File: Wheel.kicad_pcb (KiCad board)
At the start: 2 copper layers, 70.1 x 38.9 mm, 52 parts, among them J1 USB_C_Receptacle_USB2.0_16P, J2 Conn_01x06, J3 Conn_01x06, J4 Conn_01x06, J5 Conn_01x06, J6 Conn_01x03, J7 Conn_01x05, SW1 SW_Push, SW2 SW_Push, U1 STM32F407VGTx, U2 AMS1117-3.3, U3 MT6835

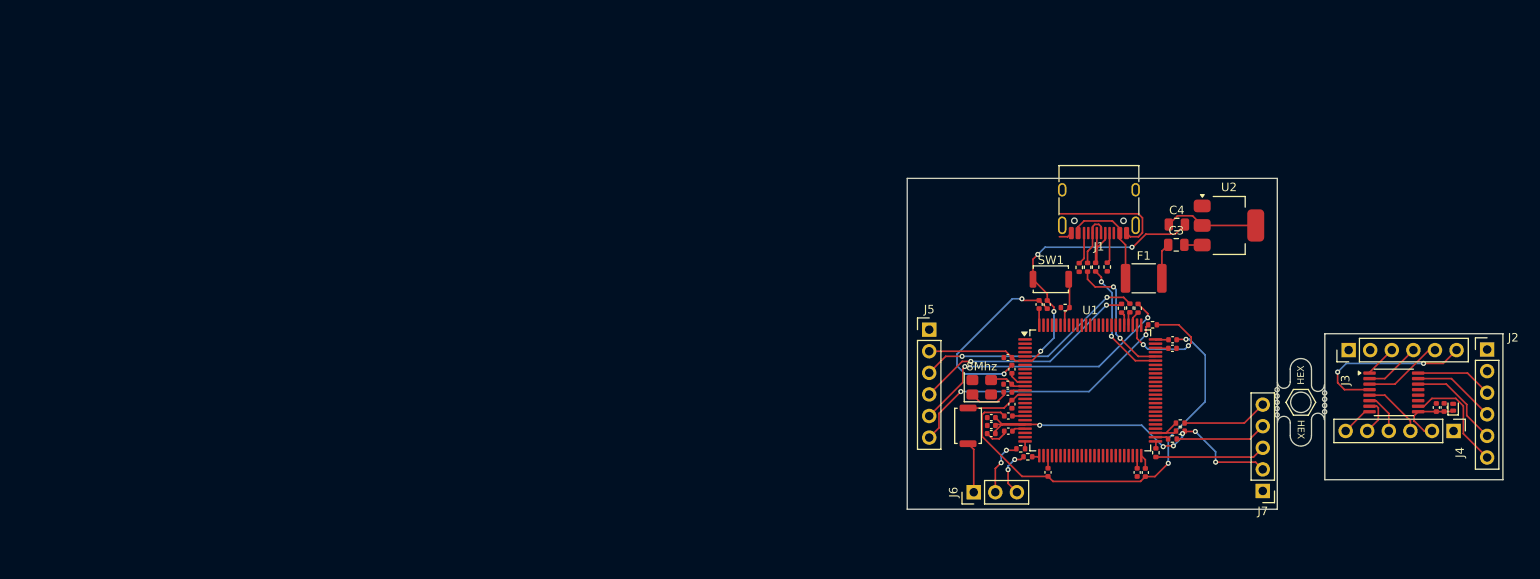
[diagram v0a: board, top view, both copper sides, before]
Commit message: Update
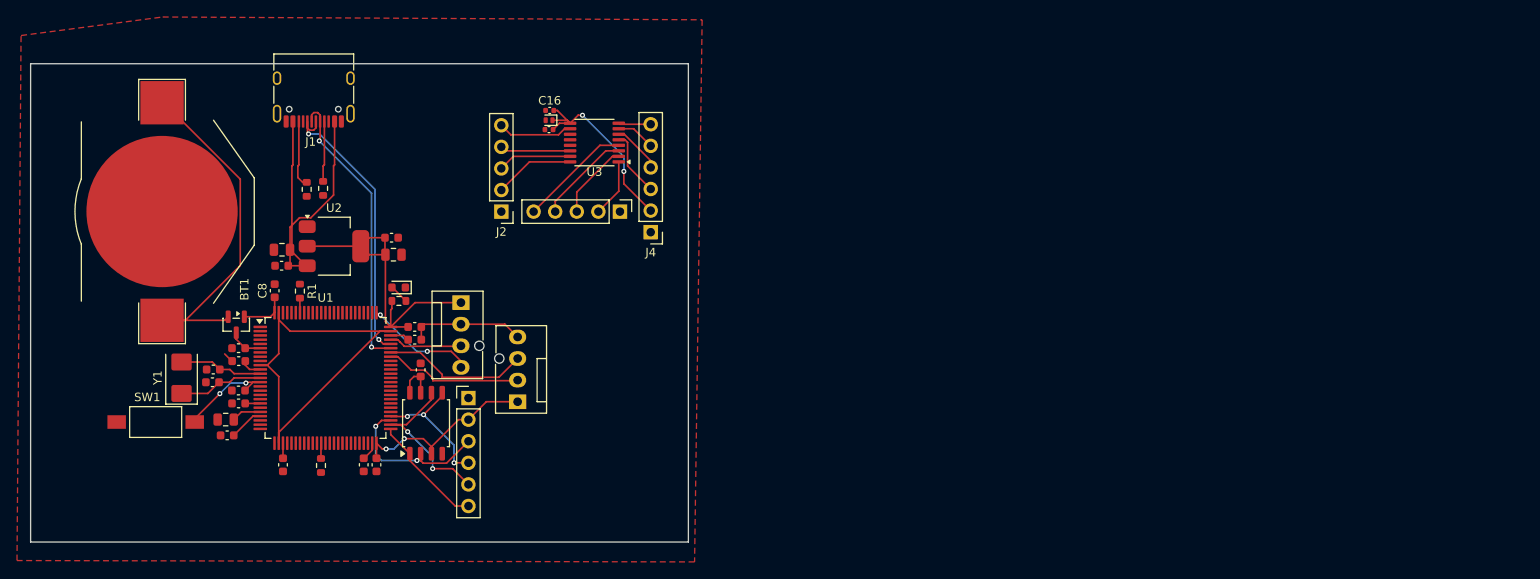
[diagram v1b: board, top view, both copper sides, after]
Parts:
- removed 8Mhz: Crystal_GND24, Crystal:Crystal_SMD_3225-4Pin_3.2x2.5mm
- removed F1: Polyfuse, Fuse:Fuse_1812_4532Metric
- removed MB5: 5.5mm, PCM_marbastlib-various:mousebites_5p5mm_easysnap
- removed R10, R11, R12, R13, R14: 100Ω, Resistor_SMD:R_0402_1005Metric
- removed R15: 10k, Resistor_SMD:R_0402_1005Metric
- removed R6, R7, R8, R9: 22Ω, Resistor_SMD:R_0402_1005Metric
- removed SW2: SW_Push, Button_Switch_SMD:SW_Push_SPST_NO_Alps_SKRK
- added BT1: Battery, Battery:BatteryHolder_Keystone_3002_1x2032, F.Cu at (77.3, 42.9)
- added D2: LED, LED_SMD:LED_0603_1608Metric, F.Cu at (105.1, 51.9)
- added D3: BAT54C, Package_TO_SOT_SMD:SOT-23, F.Cu at (86.0, 56.2)
- added U4: W25Q16JVSS, Package_SO:SOIC-8_5.3x5.3mm_P1.27mm, F.Cu at (108.3, 67.8)
- added Y1: 8MHz, Crystal:Crystal_SMD_5032-2Pin_5.0x3.2mm, F.Cu at (79.6, 62.5)
- C1, C2: value 2.2µF -> 104; footprint Capacitor_SMD:C_0402_1005Metric -> Capacitor_SMD:C_0603_1608Metric
- C10: value 100nF -> 2.2uF; footprint Capacitor_SMD:C_0402_1005Metric -> Capacitor_SMD:C_0603_1608Metric
- C11: value 4.7µF -> 2.2uF; footprint Capacitor_SMD:C_0402_1005Metric -> Capacitor_SMD:C_0603_1608Metric
- C12: value 0.1µF -> 106; footprint Capacitor_SMD:C_0402_1005Metric -> Capacitor_SMD:C_0805_2012Metric
- C13: value 27pf -> 104; footprint Capacitor_SMD:C_0402_1005Metric -> Capacitor_SMD:C_0603_1608Metric
- C14: value 27pf -> 106; footprint Capacitor_SMD:C_0402_1005Metric -> Capacitor_SMD:C_0805_2012Metric
- C17, C19: value 1µF -> 104; footprint Capacitor_SMD:C_0402_1005Metric -> Capacitor_SMD:C_0603_1608Metric
- C18: value 10nF -> 104; footprint Capacitor_SMD:C_0402_1005Metric -> Capacitor_SMD:C_0603_1608Metric
- C20: value 10nF -> 20P; footprint Capacitor_SMD:C_0402_1005Metric -> Capacitor_SMD:C_0603_1608Metric
- C21: value 100nF -> 20P; footprint Capacitor_SMD:C_0402_1005Metric -> Capacitor_SMD:C_0603_1608Metric
- C3: value 22µF -> 104; footprint Capacitor_SMD:C_0805_2012Metric -> Capacitor_SMD:C_0603_1608Metric
- C4: value 10µF -> 104; footprint Capacitor_SMD:C_0805_2012Metric -> Capacitor_SMD:C_0603_1608Metric
- C5, C6, C7, C8: value 100nF -> 104; footprint Capacitor_SMD:C_0402_1005Metric -> Capacitor_SMD:C_0603_1608Metric
- C9: value 100nF -> 106; footprint Capacitor_SMD:C_0402_1005Metric -> Capacitor_SMD:C_0805_2012Metric
- J1: value USB_C_Receptacle_USB2.0_16P -> USB_C_Receptacle_USB2.0_14P
- J2: value Conn_01x06 -> GND-A-B-Z-PWM; footprint Connector_PinHeader_2.54mm:PinHeader_1x06_P2.54mm_Vertical -> Connector_PinHeader_2.54mm:PinHeader_1x05_P2.54mm_Vertical
- J3: value Conn_01x06 -> CAL-W-V-U-GND; footprint Connector_PinHeader_2.54mm:PinHeader_1x06_P2.54mm_Vertical -> Connector_PinHeader_2.54mm:PinHeader_1x05_P2.54mm_Vertical
- J4: value Conn_01x06 -> J4(Pins 6-3)-VDDA(1)/3V3-GND
- J6: value Conn_01x03 -> Conn_01x04; footprint Connector_PinHeader_2.54mm:PinHeader_1x03_P2.54mm_Vertical -> Connector:FanPinHeader_1x04_P2.54mm_Vertical
- J7: value Conn_01x05 -> UART; footprint Connector_PinHeader_2.54mm:PinHeader_1x05_P2.54mm_Vertical -> Connector:FanPinHeader_1x04_P2.54mm_Vertical
- R1: value 5.1k -> 10k; footprint Resistor_SMD:R_0402_1005Metric -> Resistor_SMD:R_0603_1608Metric
- R2: footprint Resistor_SMD:R_0402_1005Metric -> Resistor_SMD:R_0603_1608Metric
- R3: value 20Ω -> 5.1k; footprint Resistor_SMD:R_0402_1005Metric -> Resistor_SMD:R_0603_1608Metric
- R4: value 20Ω -> 10K; footprint Resistor_SMD:R_0402_1005Metric -> Resistor_SMD:R_0603_1608Metric
- R5: value 10KΩ -> 510R; footprint Resistor_SMD:R_0402_1005Metric -> Resistor_SMD:R_0603_1608Metric
- SW1: footprint Button_Switch_SMD:SW_Push_SPST_NO_Alps_SKRK -> Button_Switch_SMD:SW_SPST_FSMSM
- moved J2 117.1 mm to (117.2, 42.9), turned to 180 degrees
- moved C4 112.4 mm to (86.3, 65.5), turned to 180 degrees
- moved C9 111.8 mm to (84.8, 67.4)
- moved D1 111.6 mm to (122.8, 32.2), turned to 180 degrees
- moved C3 111.2 mm to (86.3, 60.5), turned to 180 degrees
- moved C15 110.3 mm to (122.8, 33.3), turned to 0 degrees
- moved C16 110.0 mm to (122.9, 31.0), turned to 0 degrees
- moved SW1 106.7 mm to (76.5, 67.7)
- moved C1 106.2 mm to (86.3, 64.0), turned to 0 degrees
- moved U2 105.3 mm to (97.5, 47.0)
- moved C8 104.7 mm to (90.5, 52.2)
- moved U3 98.6 mm to (128.1, 34.8), turned to 180 degrees
- moved J4 97.3 mm to (134.8, 45.4), turned to 180 degrees
- moved C7 96.7 mm to (84.9, 69.3), turned to 180 degrees
- moved R1 95.0 mm to (93.5, 52.3)
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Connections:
- C1 pad 2: Net-(U1-VCAP_1) -> Net-(U1-NRST)
- C10 pad 1: Net-(C10-Pad1) -> GND
- C10 pad 2: Net-(C10-Pad2) -> Net-(U1-VCAP_1)
- C11 pad 1: +3V3 -> GND
- C11 pad 2: Net-(C10-Pad1) -> Net-(U1-VCAP_2)
- C12 pad 1: GND -> +5V
- C12 pad 2: Net-(U1-NRST) -> GND
- C13 pad 1: GND -> +5V
- C13 pad 2: Net-(U1-PH0) -> GND
- C14 pad 1: Net-(U1-PH1) -> VDDA(1)
- C14 pad 2: Net-(8Mhz1-Pad1) -> GND
- C15 pad 2: VCC -> VDDA(1)
- C16 pad 2: VCC -> VDDA(1)
- C17 pad 1: +3V3 -> VDDA(1)
- C18 pad 1: GND -> VBAT
- C18 pad 2: +3V3 -> GND
- C19 pad 1: Net-(C19-Pad1) -> GND
- C19 pad 2: Net-(U1-VDDA) -> Net-(U4-VCC)
- C2 pad 2: Net-(U1-VCAP_2) -> VDDA(1)
- C20 pad 1: +3V3 -> GND
- C20 pad 2: Net-(C19-Pad1) -> OSC_IN
- C21 pad 2: +3V3 -> OSC_OUT
- C3 pad 1: Net-(C3-Pad1) -> VDDA(1)
- C3 pad 2: Net-(U2-VI) -> GND
- C4 pad 1: Net-(U2-VO) -> VDDA(1)
- C4 pad 2: +3V3 -> GND
- C5 pad 1: Net-(C10-Pad1) -> VDDA(1)
- C5 pad 2: Net-(C5-Pad2) -> GND
- C6 pad 1: Net-(C10-Pad1) -> VDDA(1)
- C6 pad 2: Net-(C6-Pad2) -> GND
- C7 pad 1: Net-(C10-Pad1) -> VDDA(1)
- C7 pad 2: Net-(C7-Pad2) -> GND
- C8 pad 1: Net-(C10-Pad1) -> VDDA(1)
- C8 pad 2: Net-(C8-Pad2) -> GND
- C9 pad 1: Net-(C10-Pad1) -> VDDA(1)
- C9 pad 2: Net-(C9-Pad2) -> GND
- D1 pad 1: VCC -> VDDA(1)
- J1 pad A1: Net-(J1-GND-PadA1) -> GND
- J1 pad A12: Net-(J1-GND-PadA1) -> GND
- J1 pad A4: Net-(F1-Pad1) -> +5V
- J1 pad A6: D+ -> USB_DP
- J1 pad A7: D- -> USB_DM
- J1 pad A8: unconnected-(J1-SBU1-PadA8) -> (no net)
- J1 pad A9: Net-(F1-Pad1) -> +5V
- J1 pad B1: Net-(J1-GND-PadA1) -> GND
- J1 pad B12: Net-(J1-GND-PadA1) -> GND
- J1 pad B4: Net-(F1-Pad1) -> +5V
- J1 pad B6: D+ -> USB_DP
- J1 pad B7: D- -> USB_DM
- J1 pad B8: unconnected-(J1-SBU2-PadB8) -> (no net)
- J1 pad B9: Net-(F1-Pad1) -> +5V
- J1 pad SH: unconnected-(J1-SHIELD-PadSH) -> GND
- J2 pad 2: VCC -> A
- J2 pad 3: A -> B
- J2 pad 4: B -> Z
- J2 pad 5: Z -> PWM
- J3 pad 2: VCC -> U
- J3 pad 3: U -> V
- J3 pad 4: V -> W
- J3 pad 5: W -> CAL
- J4 pad 2: VCC -> VDDA(1)
- J5 pad 2: +3V3 -> VDDA(1)
- J5 pad 3: Net-(J5-Pin_3) -> MISO
- J5 pad 4: Net-(J5-Pin_4) -> MOSI
- J5 pad 5: Net-(J5-Pin_5) -> SCK
- J5 pad 6: Net-(J5-Pin_6) -> CS
- J6 pad 1: GND -> VDDA(1)
- J6 pad 2: HOV_TX -> GND
- J6 pad 3: HOV_RX -> Net-(J6-Pin_3)
- J7 pad 1: GND -> VDDA(1)
- J7 pad 2: +3V3 -> TX_OUT
- J7 pad 3: Net-(J7-Pin_3) -> RX_IN
- J7 pad 4: Net-(J7-Pin_4) -> GND
- R1 pad 1: Net-(J1-CC1) -> GND
- R1 pad 2: GND -> Net-(U1-BOOT0)
- R2 pad 1: Net-(J1-CC2) -> Net-(J1-CC1)
- R3 pad 1: Net-(U1-PA11) -> Net-(J1-CC2)
- R3 pad 2: D- -> GND
- R4 pad 1: Net-(U1-PA12) -> Net-(U1-PB2)
- R4 pad 2: D+ -> GND
- R5 pad 1: Net-(U1-BOOT0) -> VDDA(1)
- R5 pad 2: GND -> Net-(D2-A)
- SW1 pad 1: +3V3 -> GND
- SW1 pad 2: Net-(U1-BOOT0) -> Net-(U1-NRST)
- U1 pad 100: Net-(C10-Pad2) -> VDDA(1)
- U1 pad 11: Net-(C5-Pad2) -> VDDA(1)
- U1 pad 12: Net-(U1-PH0) -> OSC_IN
- U1 pad 13: Net-(U1-PH1) -> OSC_OUT
- U1 pad 19: Net-(C6-Pad2) -> VDDA(1)
- U1 pad 20: GND -> unconnected-(U1-VSSA-Pad20)
- U1 pad 21: +3V3 -> VDDA(1)
- U1 pad 22: Net-(U1-VDDA) -> VDDA(1)
- U1 pad 25: Net-(U1-PA2) -> unconnected-(U1-PA2-Pad25)
- U1 pad 26: Net-(U1-PA3) -> unconnected-(U1-PA3-Pad26)
- U1 pad 28: Net-(C7-Pad2) -> VDDA(1)
- U1 pad 37: unconnected-(U1-PB2-Pad37) -> Net-(U1-PB2)
- U1 pad 50: Net-(C8-Pad2) -> VDDA(1)
- U1 pad 51: LATCH/CS -> CS
- U1 pad 52: SCK(S) -> SCK
- U1 pad 53: MISO(S) -> MISO
- U1 pad 54: unconnected-(U1-PB15-Pad54) -> MOSI
- U1 pad 6: +3V3 -> VBAT
- U1 pad 68: unconnected-(U1-PA9-Pad68) -> TX_OUT
- U1 pad 69: unconnected-(U1-PA10-Pad69) -> RX_IN
- U1 pad 70: Net-(U1-PA11) -> USB_DM
- U1 pad 71: Net-(U1-PA12) -> USB_DP
- U1 pad 72: unconnected-(U1-PA13-Pad72) -> Net-(J6-Pin_3)
- U1 pad 75: Net-(C9-Pad2) -> VDDA(1)
- U1 pad 76: unconnected-(U1-PA14-Pad76) -> Net-(J6-Pin_4)
- U1 pad 77: CSN -> unconnected-(U1-PA15-Pad77)
- U1 pad 78: SCK -> unconnected-(U1-PC10-Pad78)
- U1 pad 79: MISO -> unconnected-(U1-PC11-Pad79)
- U1 pad 80: MOSI -> unconnected-(U1-PC12-Pad80)
- U2 pad 2: Net-(U2-VO) -> VDDA(1)
- U2 pad 3: Net-(U2-VI) -> +5V
- U3 pad 9: VCC -> VDDA(1)
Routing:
- net VDDA(1): track 0.00 -> 103.4 mm, vias 0 -> 4
- net +3V3: track 90.3 -> 0.00 mm, vias 10 -> 0
- net Net-(C10-Pad1): track 71.6 -> 0.00 mm, vias 4 -> 0
- net GND: track 5.99 -> 66.0 mm
- net Net-(BT1-+): track 0.00 -> 43.1 mm
- net +5V: track 0.00 -> 40.3 mm
- net USB_DP: track 0.00 -> 34.2 mm, vias 0 -> 2
- net USB_DM: track 0.00 -> 34.2 mm, vias 0 -> 2
- net Net-(J5-Pin_5): track 33.6 -> 0.00 mm, vias 2 -> 0
- net Net-(J5-Pin_6): track 32.8 -> 0.00 mm, vias 2 -> 0
- net Net-(J5-Pin_3): track 27.6 -> 0.00 mm, vias 2 -> 0
- net Net-(J5-Pin_4): track 27.0 -> 0.00 mm, vias 2 -> 0
- net SCK: track 1.75 -> 19.7 mm, vias 0 -> 2
- net MISO: track 1.58 -> 19.1 mm, vias 0 -> 2
- net RX_IN: track 0.00 -> 17.3 mm
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- added copper zone on F.Cu, net GND
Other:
- board size 70.1 x 38.9 mm -> 77.4 x 56.3 mm
